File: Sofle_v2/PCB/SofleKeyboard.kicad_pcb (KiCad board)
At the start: 2 copper layers, 143.5 x 115.5 mm, 89 parts, among them J1 LED, J2 4PIN, J3 OLED, SW1 SW_PUSH, SW10 SW_PUSH, SW11 SW_PUSH, SW12 SW_PUSH, SW13 SW_PUSH, SW14 SW_PUSH, SW15 SW_PUSH, SW16 SW_PUSH, SW17 SW_PUSH, SW18 SW_PUSH, SW19 SW_PUSH, SW2 SW_PUSH, SW20 SW_PUSH, SW21 SW_PUSH, SW22 SW_PUSH, SW23 SW_PUSH, SW24 SW_PUSH, SW25 Rotary_Encoder_Switch, SW26 SW_PUSH, SW27 SW_PUSH, SW28 SW_PUSH, SW29 SW_PUSH, SW3 SW_PUSH, SW30 SW_PUSH, SW4 SW_PUSH, SW5 SW_PUSH, SW6 SW_PUSH, SW7 SW_PUSH, SW8 SW_PUSH, SW9 SW_PUSH, U1 ProMicro

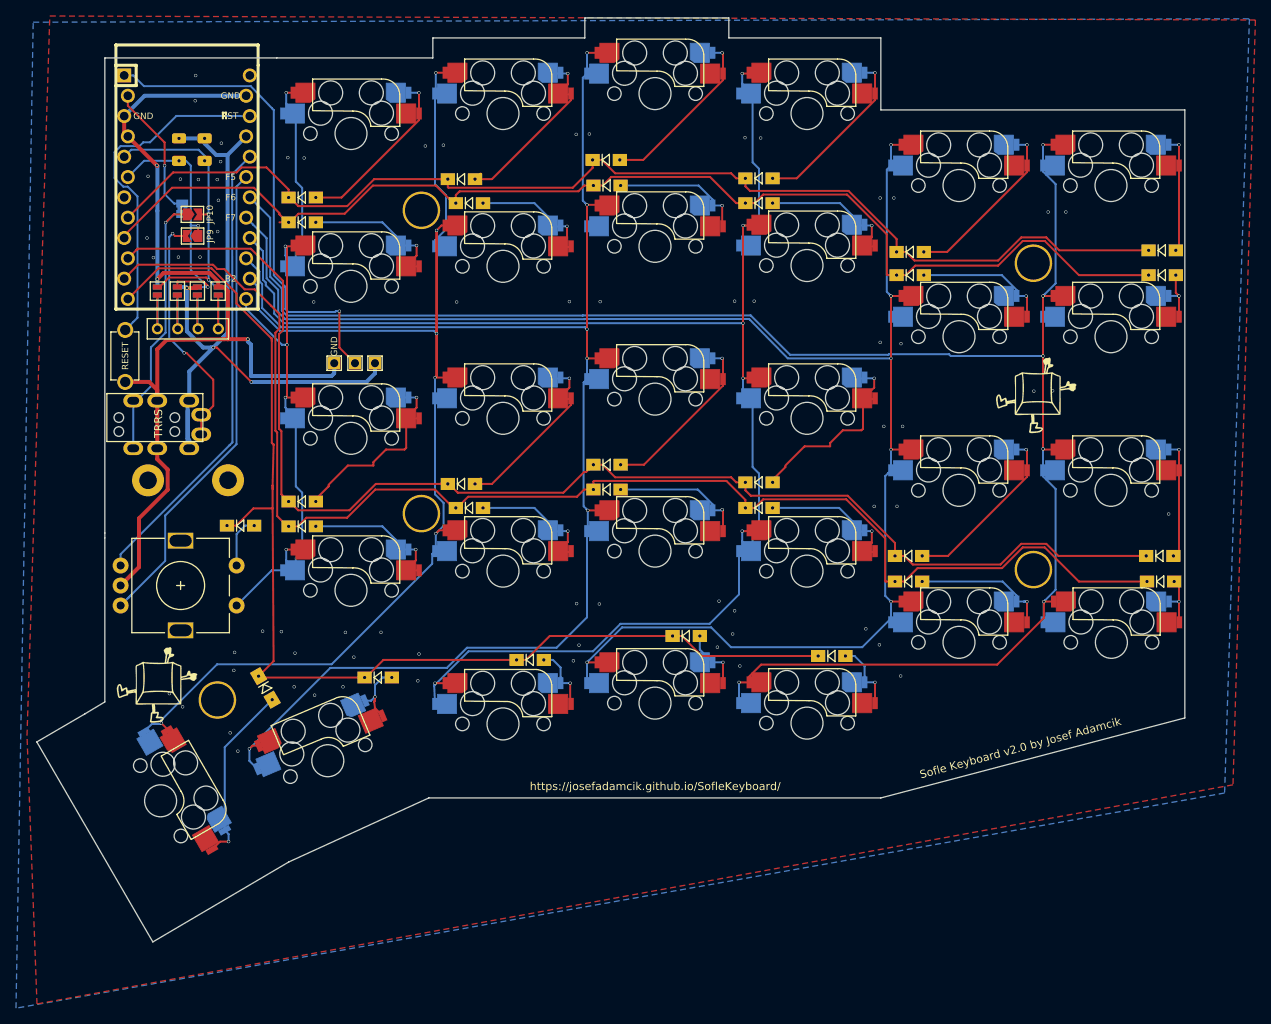
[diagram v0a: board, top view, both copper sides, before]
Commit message: Work on Sofle Wireless Added footprints Placement of footprints
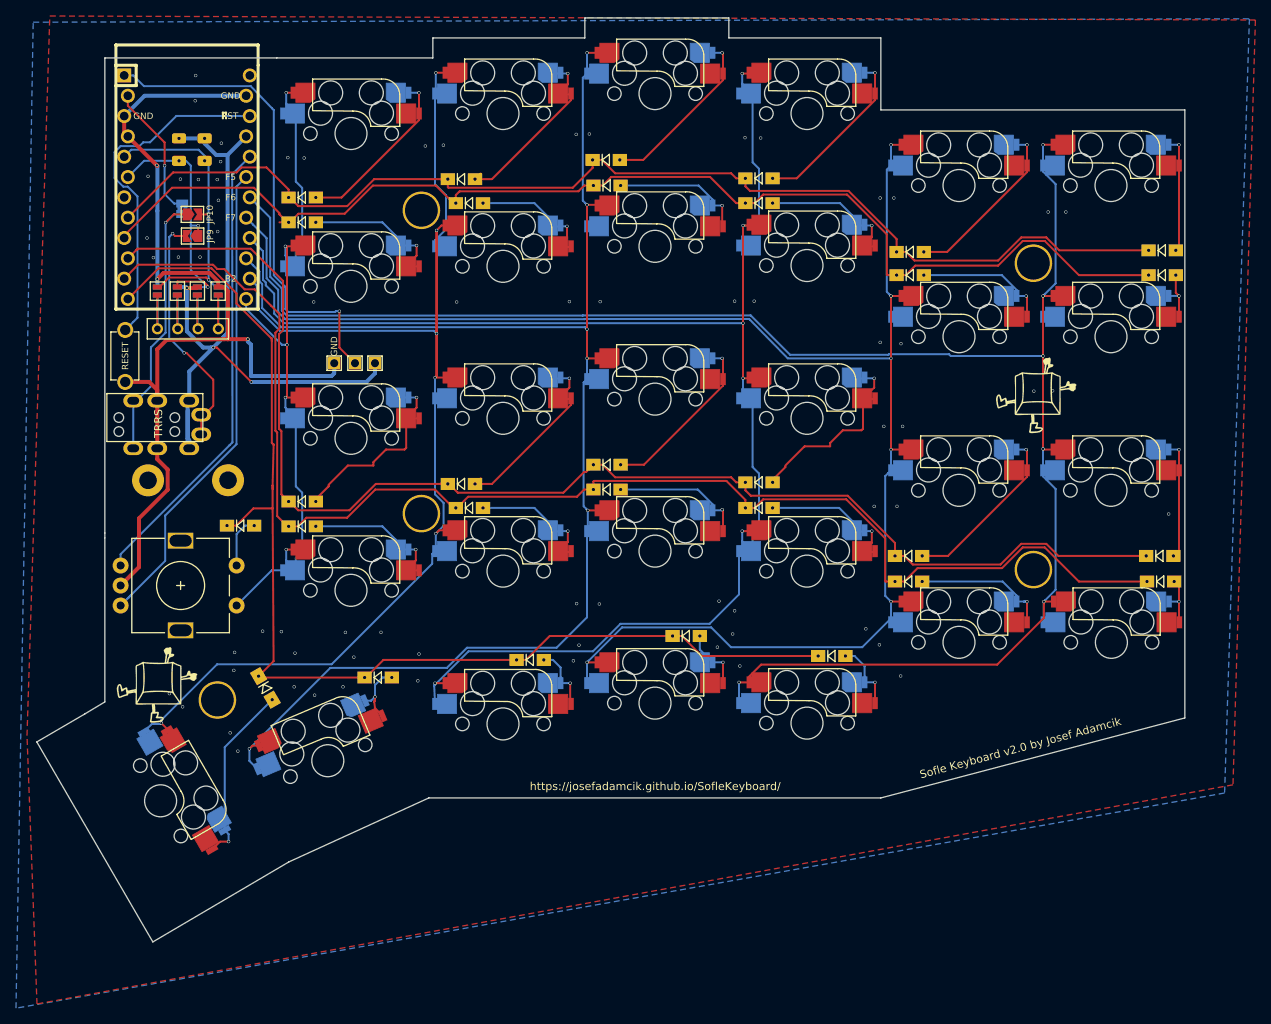
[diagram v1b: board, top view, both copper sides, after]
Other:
- net class Default removed
- net class GND removed
- net class VCC removed
